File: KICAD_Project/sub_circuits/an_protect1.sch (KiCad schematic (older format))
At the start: 20 parts

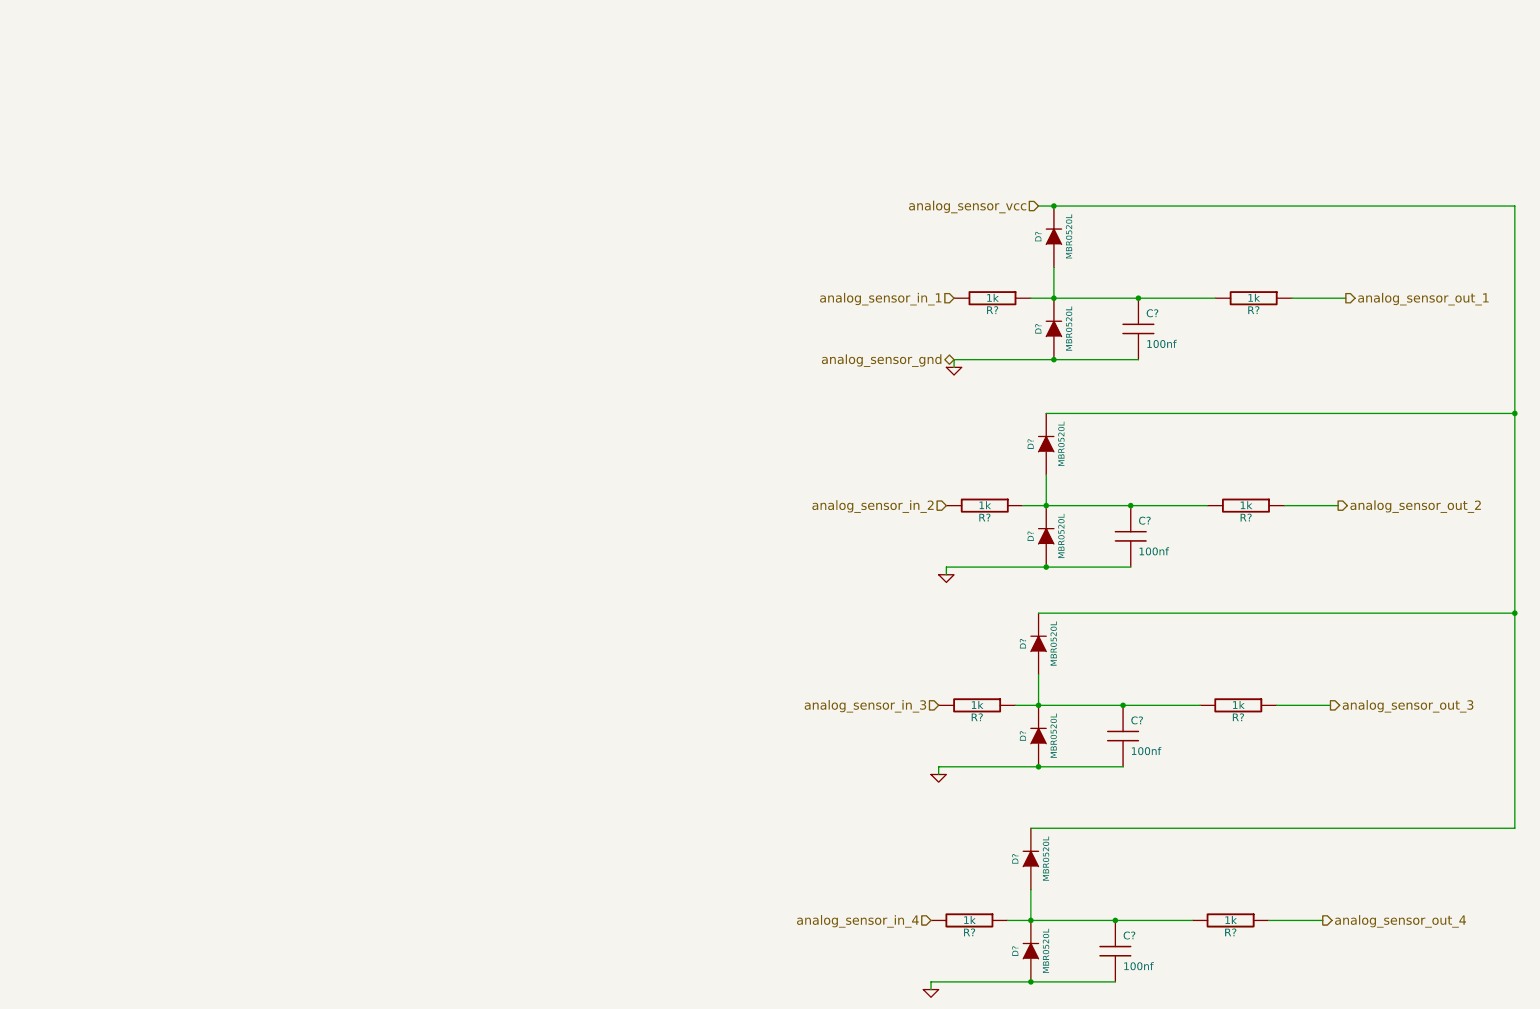
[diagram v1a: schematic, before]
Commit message: About to runs scripts to scrub the BOM's, so here's a backup copy in case it goes wrong.
Signed-off-by: Jared Harvey <TortiseGIT@jaredharvey.com>
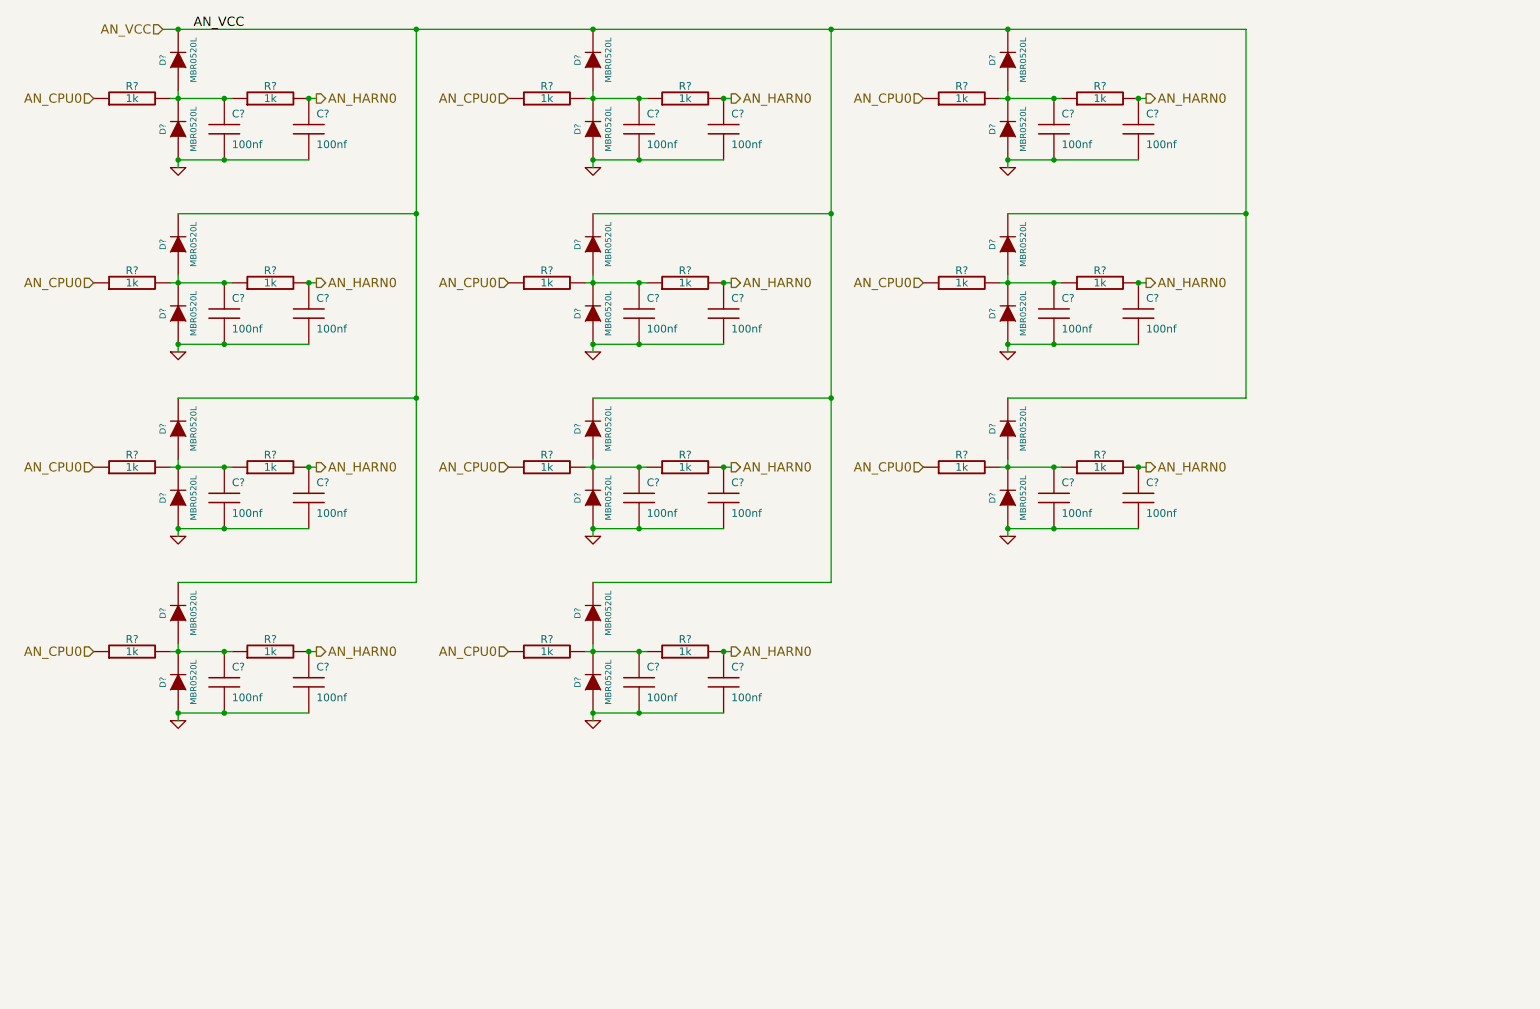
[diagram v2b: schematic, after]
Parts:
- removed C? (x4): 100nf, SM0805-C1, symbol C
- removed D? (x8): MBR0520L, SOD123, symbol DIODE
- removed R? (x8): 1k, SM0805-R4, symbol R
- added C? (x22): 100nf, SM0805-C1, symbol C
- added D? (x22): MBR0520L, SOD123, symbol DIODE
- added R? (x22): 1k, SM0805, symbol R
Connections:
- net GND: now also C?.2, C?.2, C?.2, C?.2, C?.2, C?.2, C?.2, C?.2, C?.2, C?.2, C?.2, C?.2, C?.2, C?.2, C?.2, C?.2, C?.2, C?.2, C?.2, C?.2, C?.2, C?.2, D?.1 (A), D?.1 (A), D?.1 (A), D?.1 (A), D?.1 (A), D?.1 (A), D?.1 (A), D?.1 (A), D?.1 (A), D?.1 (A), D?.1 (A)
- new net: C?.1, D?.1 (A), D?.2 (K), R?.1, R?.2 (x11)
- new net AN_CPU0: R?.1, R?.1, R?.1, R?.1, R?.1, R?.1, R?.1, R?.1, R?.1, R?.1, R?.1
- new net AN_HARN0: C?.1, C?.1, C?.1, C?.1, C?.1, C?.1, C?.1, C?.1, C?.1, C?.1, C?.1, R?.2, R?.2, R?.2, R?.2, R?.2, R?.2, R?.2, R?.2, R?.2, R?.2, R?.2
- new net AN_VCC: D?.2 (K), D?.2 (K), D?.2 (K), D?.2 (K), D?.2 (K), D?.2 (K), D?.2 (K), D?.2 (K), D?.2 (K), D?.2 (K), D?.2 (K)

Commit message: caps have been done with the scripts next up is the resistors.
Signed-off-by: Jared Harvey <TortiseGIT@jaredharvey.com>
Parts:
- C? (x22): Field3 -,- -> (none); Field4 -,- -> (none); Field5 50,V -> (none); Field6 10,% -> (none); Field7 Ceramic -> (none); Field8 other,more,stuff -> (none); V (none) -> 100V; construct (none) -> ceramic; mfg,# avx,08055F102K4Z2A -> (none); mfg,mfg# (none) -> avx,08051C104KAT2A; misc (none) -> other,more,stuff; tolerance (none) -> 10%; vend,# newark,26M5154 -> (none); vend1,vend1# (none) -> newark,96M1354

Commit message: Looks like the bulk components are golden now, there are still a couple straglers, mostly switch mode power supply stuff.
Signed-off-by: Jared Harvey <TortiseGIT@jaredharvey.com>
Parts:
- R? (x22): Field1 vishay,CRCW08051K00FKTA -> (none); Field2 newark,05F1507 -> (none); Field3 -,- -> (none); Field4 -,- -> (none); Field5 125,mW -> (none); Field6 1,% -> (none); Field7 thick film -> (none); Field8 other,more,stuff -> (none); construct (none) -> thick film; mfg,mfg# (none) -> vishay,CRCW08051K00FKTA; misc (none) -> other,more,stuff; tolerance (none) -> 1%; vend1,vend1# (none) -> newark,05F1507; w (none) -> 125mW

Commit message: More work on footprints, and schematic BOM's.
Signed-off-by: Jared Harvey <TortiseGIT@jaredharvey.com>
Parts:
- R? (x22): W (none) -> 125mW; tol (none) -> 1%; tolerance 1% -> (none); w 125mW -> (none)
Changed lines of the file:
@@
 F 6 "" V 1130 2600 60  0001 C CNN ""
 F 7 "" V 1130 2600 60  0001 C CNN ""
-F 8 "125mW" V 1130 2600 60  0001 C CNN "w"
-F 9 "1%" V 1130 2600 60  0001 C CNN "tolerance"
+F 8 "125mW" V 1130 2600 60  0001 C CNN "W"
+F 9 "1%" V 1130 2600 60  0001 C CNN "tol"
 F 10 "thick film" V 1130 2600 60  0001 C CNN "construct"
 F 11 "other,more,stuff" V 1130 2600 60  0001 C CNN "misc"
@@
 F 6 "" V 1130 2600 60  0001 C CNN ""
 F 7 "" V 1130 2600 60  0001 C CNN ""
-F 8 "125mW" V 1130 2600 60  0001 C CNN "w"
-F 9 "1%" V 1130 2600 60  0001 C CNN "tolerance"
+F 8 "125mW" V 1130 2600 60  0001 C CNN "W"
+F 9 "1%" V 1130 2600 60  0001 C CNN "tol"
 F 10 "thick film" V 1130 2600 60  0001 C CNN "construct"
 F 11 "other,more,stuff" V 1130 2600 60  0001 C CNN "misc"
@@
 F 6 "" V 1130 2600 60  0001 C CNN ""
 F 7 "" V 1130 2600 60  0001 C CNN ""
-F 8 "125mW" V 1130 2600 60  0001 C CNN "w"
-F 9 "1%" V 1130 2600 60  0001 C CNN "tolerance"
+F 8 "125mW" V 1130 2600 60  0001 C CNN "W"
+F 9 "1%" V 1130 2600 60  0001 C CNN "tol"
 F 10 "thick film" V 1130 2600 60  0001 C CNN "construct"
 F 11 "other,more,stuff" V 1130 2600 60  0001 C CNN "misc"
@@
 F 6 "" V 1130 2600 60  0001 C CNN ""
 F 7 "" V 1130 2600 60  0001 C CNN ""
-F 8 "125mW" V 1130 2600 60  0001 C CNN "w"
-F 9 "1%" V 1130 2600 60  0001 C CNN "tolerance"
+F 8 "125mW" V 1130 2600 60  0001 C CNN "W"
+F 9 "1%" V 1130 2600 60  0001 C CNN "tol"
 F 10 "thick film" V 1130 2600 60  0001 C CNN "construct"
 F 11 "other,more,stuff" V 1130 2600 60  0001 C CNN "misc"
@@
 F 6 "" V 1130 2600 60  0001 C CNN ""
 F 7 "" V 1130 2600 60  0001 C CNN ""
-F 8 "125mW" V 1130 2600 60  0001 C CNN "w"
-F 9 "1%" V 1130 2600 60  0001 C CNN "tolerance"
+F 8 "125mW" V 1130 2600 60  0001 C CNN "W"
+F 9 "1%" V 1130 2600 60  0001 C CNN "tol"
 F 10 "thick film" V 1130 2600 60  0001 C CNN "construct"
 F 11 "other,more,stuff" V 1130 2600 60  0001 C CNN "misc"
@@
 F 6 "" V 1130 2600 60  0001 C CNN ""
 F 7 "" V 1130 2600 60  0001 C CNN ""
-F 8 "125mW" V 1130 2600 60  0001 C CNN "w"
-F 9 "1%" V 1130 2600 60  0001 C CNN "tolerance"
+F 8 "125mW" V 1130 2600 60  0001 C CNN "W"
+F 9 "1%" V 1130 2600 60  0001 C CNN "tol"
 F 10 "thick film" V 1130 2600 60  0001 C CNN "construct"
 F 11 "other,more,stuff" V 1130 2600 60  0001 C CNN "misc"
@@
 F 6 "" V 1130 2600 60  0001 C CNN ""
 F 7 "" V 1130 2600 60  0001 C CNN ""
-F 8 "125mW" V 1130 2600 60  0001 C CNN "w"
-F 9 "1%" V 1130 2600 60  0001 C CNN "tolerance"
+F 8 "125mW" V 1130 2600 60  0001 C CNN "W"
+F 9 "1%" V 1130 2600 60  0001 C CNN "tol"
 F 10 "thick film" V 1130 2600 60  0001 C CNN "construct"
 F 11 "other,more,stuff" V 1130 2600 60  0001 C CNN "misc"
@@
 F 6 "" V 1130 2600 60  0001 C CNN ""
 F 7 "" V 1130 2600 60  0001 C CNN ""
-F 8 "125mW" V 1130 2600 60  0001 C CNN "w"
-F 9 "1%" V 1130 2600 60  0001 C CNN "tolerance"
+F 8 "125mW" V 1130 2600 60  0001 C CNN "W"
+F 9 "1%" V 1130 2600 60  0001 C CNN "tol"
 F 10 "thick film" V 1130 2600 60  0001 C CNN "construct"
 F 11 "other,more,stuff" V 1130 2600 60  0001 C CNN "misc"
@@
 F 6 "" V 1130 2600 60  0001 C CNN ""
 F 7 "" V 1130 2600 60  0001 C CNN ""
-F 8 "125mW" V 1130 2600 60  0001 C CNN "w"
-F 9 "1%" V 1130 2600 60  0001 C CNN "tolerance"
+F 8 "125mW" V 1130 2600 60  0001 C CNN "W"
+F 9 "1%" V 1130 2600 60  0001 C CNN "tol"
 F 10 "thick film" V 1130 2600 60  0001 C CNN "construct"
 F 11 "other,more,stuff" V 1130 2600 60  0001 C CNN "misc"
@@
 F 6 "" V 1130 2600 60  0001 C CNN ""
 F 7 "" V 1130 2600 60  0001 C CNN ""
-F 8 "125mW" V 1130 2600 60  0001 C CNN "w"
-F 9 "1%" V 1130 2600 60  0001 C CNN "tolerance"
+F 8 "125mW" V 1130 2600 60  0001 C CNN "W"
+F 9 "1%" V 1130 2600 60  0001 C CNN "tol"
 F 10 "thick film" V 1130 2600 60  0001 C CNN "construct"
 F 11 "other,more,stuff" V 1130 2600 60  0001 C CNN "misc"
@@
 F 6 "" V 1130 2600 60  0001 C CNN ""
 F 7 "" V 1130 2600 60  0001 C CNN ""
-F 8 "125mW" V 1130 2600 60  0001 C CNN "w"
-F 9 "1%" V 1130 2600 60  0001 C CNN "tolerance"
+F 8 "125mW" V 1130 2600 60  0001 C CNN "W"
+F 9 "1%" V 1130 2600 60  0001 C CNN "tol"
 F 10 "thick film" V 1130 2600 60  0001 C CNN "construct"
 F 11 "other,more,stuff" V 1130 2600 60  0001 C CNN "misc"
@@
 F 6 "" V 1130 2600 60  0001 C CNN ""
 F 7 "" V 1130 2600 60  0001 C CNN ""
-F 8 "125mW" V 1130 2600 60  0001 C CNN "w"
-F 9 "1%" V 1130 2600 60  0001 C CNN "tolerance"
+F 8 "125mW" V 1130 2600 60  0001 C CNN "W"
+F 9 "1%" V 1130 2600 60  0001 C CNN "tol"
 F 10 "thick film" V 1130 2600 60  0001 C CNN "construct"
 F 11 "other,more,stuff" V 1130 2600 60  0001 C CNN "misc"
@@
 F 6 "" V 1130 2600 60  0001 C CNN ""
 F 7 "" V 1130 2600 60  0001 C CNN ""
-F 8 "125mW" V 1130 2600 60  0001 C CNN "w"
-F 9 "1%" V 1130 2600 60  0001 C CNN "tolerance"
+F 8 "125mW" V 1130 2600 60  0001 C CNN "W"
+F 9 "1%" V 1130 2600 60  0001 C CNN "tol"
 F 10 "thick film" V 1130 2600 60  0001 C CNN "construct"
 F 11 "other,more,stuff" V 1130 2600 60  0001 C CNN "misc"
@@
 F 6 "" V 1130 2600 60  0001 C CNN ""
 F 7 "" V 1130 2600 60  0001 C CNN ""
-F 8 "125mW" V 1130 2600 60  0001 C CNN "w"
-F 9 "1%" V 1130 2600 60  0001 C CNN "tolerance"
+F 8 "125mW" V 1130 2600 60  0001 C CNN "W"
+F 9 "1%" V 1130 2600 60  0001 C CNN "tol"
 F 10 "thick film" V 1130 2600 60  0001 C CNN "construct"
 F 11 "other,more,stuff" V 1130 2600 60  0001 C CNN "misc"
@@
 F 6 "" V 1130 2600 60  0001 C CNN ""
 F 7 "" V 1130 2600 60  0001 C CNN ""
-F 8 "125mW" V 1130 2600 60  0001 C CNN "w"
-F 9 "1%" V 1130 2600 60  0001 C CNN "tolerance"
+F 8 "125mW" V 1130 2600 60  0001 C CNN "W"
+F 9 "1%" V 1130 2600 60  0001 C CNN "tol"
 F 10 "thick film" V 1130 2600 60  0001 C CNN "construct"
 F 11 "other,more,stuff" V 1130 2600 60  0001 C CNN "misc"
@@
 F 6 "" V 1130 2600 60  0001 C CNN ""
 F 7 "" V 1130 2600 60  0001 C CNN ""
-F 8 "125mW" V 1130 2600 60  0001 C CNN "w"
-F 9 "1%" V 1130 2600 60  0001 C CNN "tolerance"
+F 8 "125mW" V 1130 2600 60  0001 C CNN "W"
+F 9 "1%" V 1130 2600 60  0001 C CNN "tol"
 F 10 "thick film" V 1130 2600 60  0001 C CNN "construct"
 F 11 "other,more,stuff" V 1130 2600 60  0001 C CNN "misc"
@@
 F 6 "" V 1130 2600 60  0001 C CNN ""
 F 7 "" V 1130 2600 60  0001 C CNN ""
-F 8 "125mW" V 1130 2600 60  0001 C CNN "w"
-F 9 "1%" V 1130 2600 60  0001 C CNN "tolerance"
+F 8 "125mW" V 1130 2600 60  0001 C CNN "W"
+F 9 "1%" V 1130 2600 60  0001 C CNN "tol"
 F 10 "thick film" V 1130 2600 60  0001 C CNN "construct"
 F 11 "other,more,stuff" V 1130 2600 60  0001 C CNN "misc"
@@
 F 6 "" V 1130 2600 60  0001 C CNN ""
 F 7 "" V 1130 2600 60  0001 C CNN ""
-F 8 "125mW" V 1130 2600 60  0001 C CNN "w"
-F 9 "1%" V 1130 2600 60  0001 C CNN "tolerance"
+F 8 "125mW" V 1130 2600 60  0001 C CNN "W"
+F 9 "1%" V 1130 2600 60  0001 C CNN "tol"
 F 10 "thick film" V 1130 2600 60  0001 C CNN "construct"
 F 11 "other,more,stuff" V 1130 2600 60  0001 C CNN "misc"
@@
 F 6 "" V 1130 2600 60  0001 C CNN ""
 F 7 "" V 1130 2600 60  0001 C CNN ""
-F 8 "125mW" V 1130 2600 60  0001 C CNN "w"
-F 9 "1%" V 1130 2600 60  0001 C CNN "tolerance"
+F 8 "125mW" V 1130 2600 60  0001 C CNN "W"
+F 9 "1%" V 1130 2600 60  0001 C CNN "tol"
 F 10 "thick film" V 1130 2600 60  0001 C CNN "construct"
 F 11 "other,more,stuff" V 1130 2600 60  0001 C CNN "misc"
@@
 F 6 "" V 1130 2600 60  0001 C CNN ""
 F 7 "" V 1130 2600 60  0001 C CNN ""
-F 8 "125mW" V 1130 2600 60  0001 C CNN "w"
-F 9 "1%" V 1130 2600 60  0001 C CNN "tolerance"
+F 8 "125mW" V 1130 2600 60  0001 C CNN "W"
+F 9 "1%" V 1130 2600 60  0001 C CNN "tol"
 F 10 "thick film" V 1130 2600 60  0001 C CNN "construct"
 F 11 "other,more,stuff" V 1130 2600 60  0001 C CNN "misc"
@@
 F 6 "" V 1130 2600 60  0001 C CNN ""
 F 7 "" V 1130 2600 60  0001 C CNN ""
-F 8 "125mW" V 1130 2600 60  0001 C CNN "w"
-F 9 "1%" V 1130 2600 60  0001 C CNN "tolerance"
+F 8 "125mW" V 1130 2600 60  0001 C CNN "W"
+F 9 "1%" V 1130 2600 60  0001 C CNN "tol"
 F 10 "thick film" V 1130 2600 60  0001 C CNN "construct"
 F 11 "other,more,stuff" V 1130 2600 60  0001 C CNN "misc"
@@
 F 6 "" V 1130 2600 60  0001 C CNN ""
 F 7 "" V 1130 2600 60  0001 C CNN ""
-F 8 "125mW" V 1130 2600 60  0001 C CNN "w"
-F 9 "1%" V 1130 2600 60  0001 C CNN "tolerance"
-F 10 "thick film" V 1130 2600 60  0001 C CNN "construct"
-F 11 "other,more,stuff" V 1130 2600 60  0001 C CNN "misc"
+F 8 "125mW" V 1130 2600 60  0001 C CNN "W"
+F 9 "1%" V 1130 2600 60  0001 C CNN "tol"
+F 10 "thick film" V 1130 2600 60  0001 C CNN "construct"
+F 11 "other,more,stuff" V 1130 2600 60  0001 C CNN "misc"
